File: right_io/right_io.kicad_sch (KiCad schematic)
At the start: 0 parts

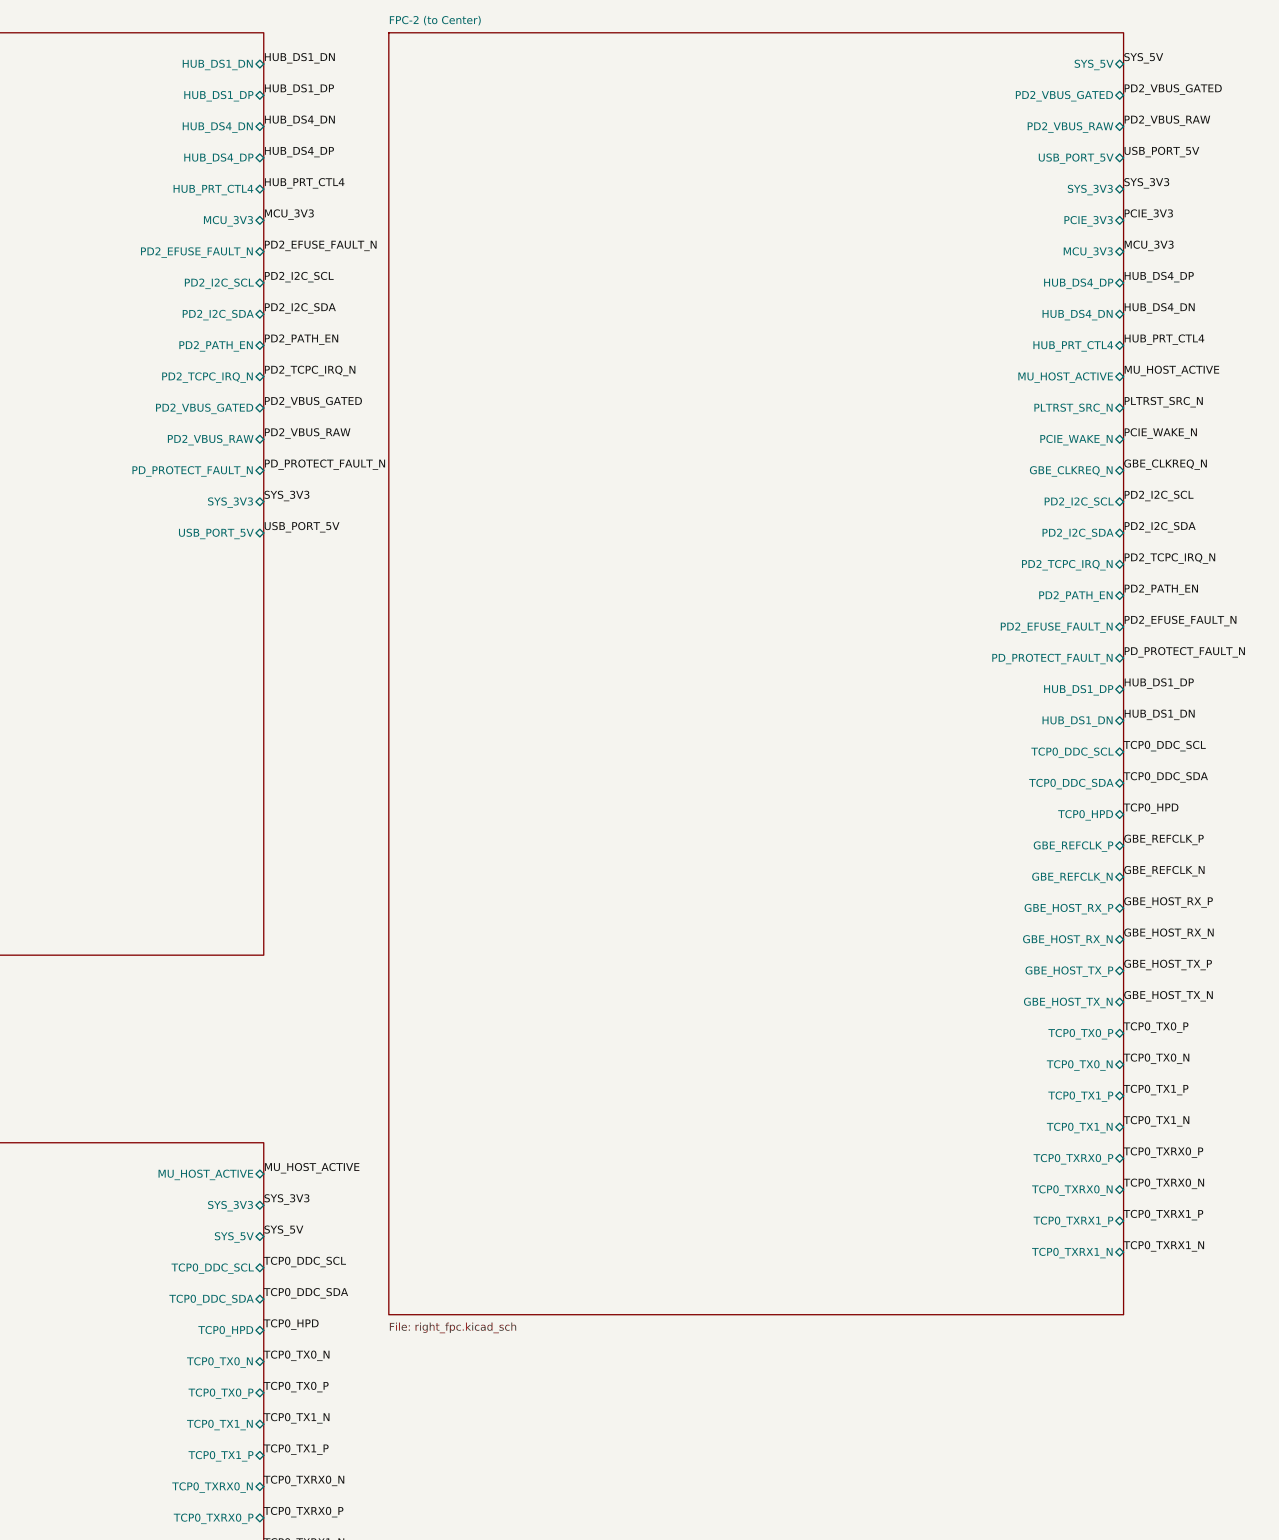
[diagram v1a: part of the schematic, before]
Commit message: fix the center layout and more board issues
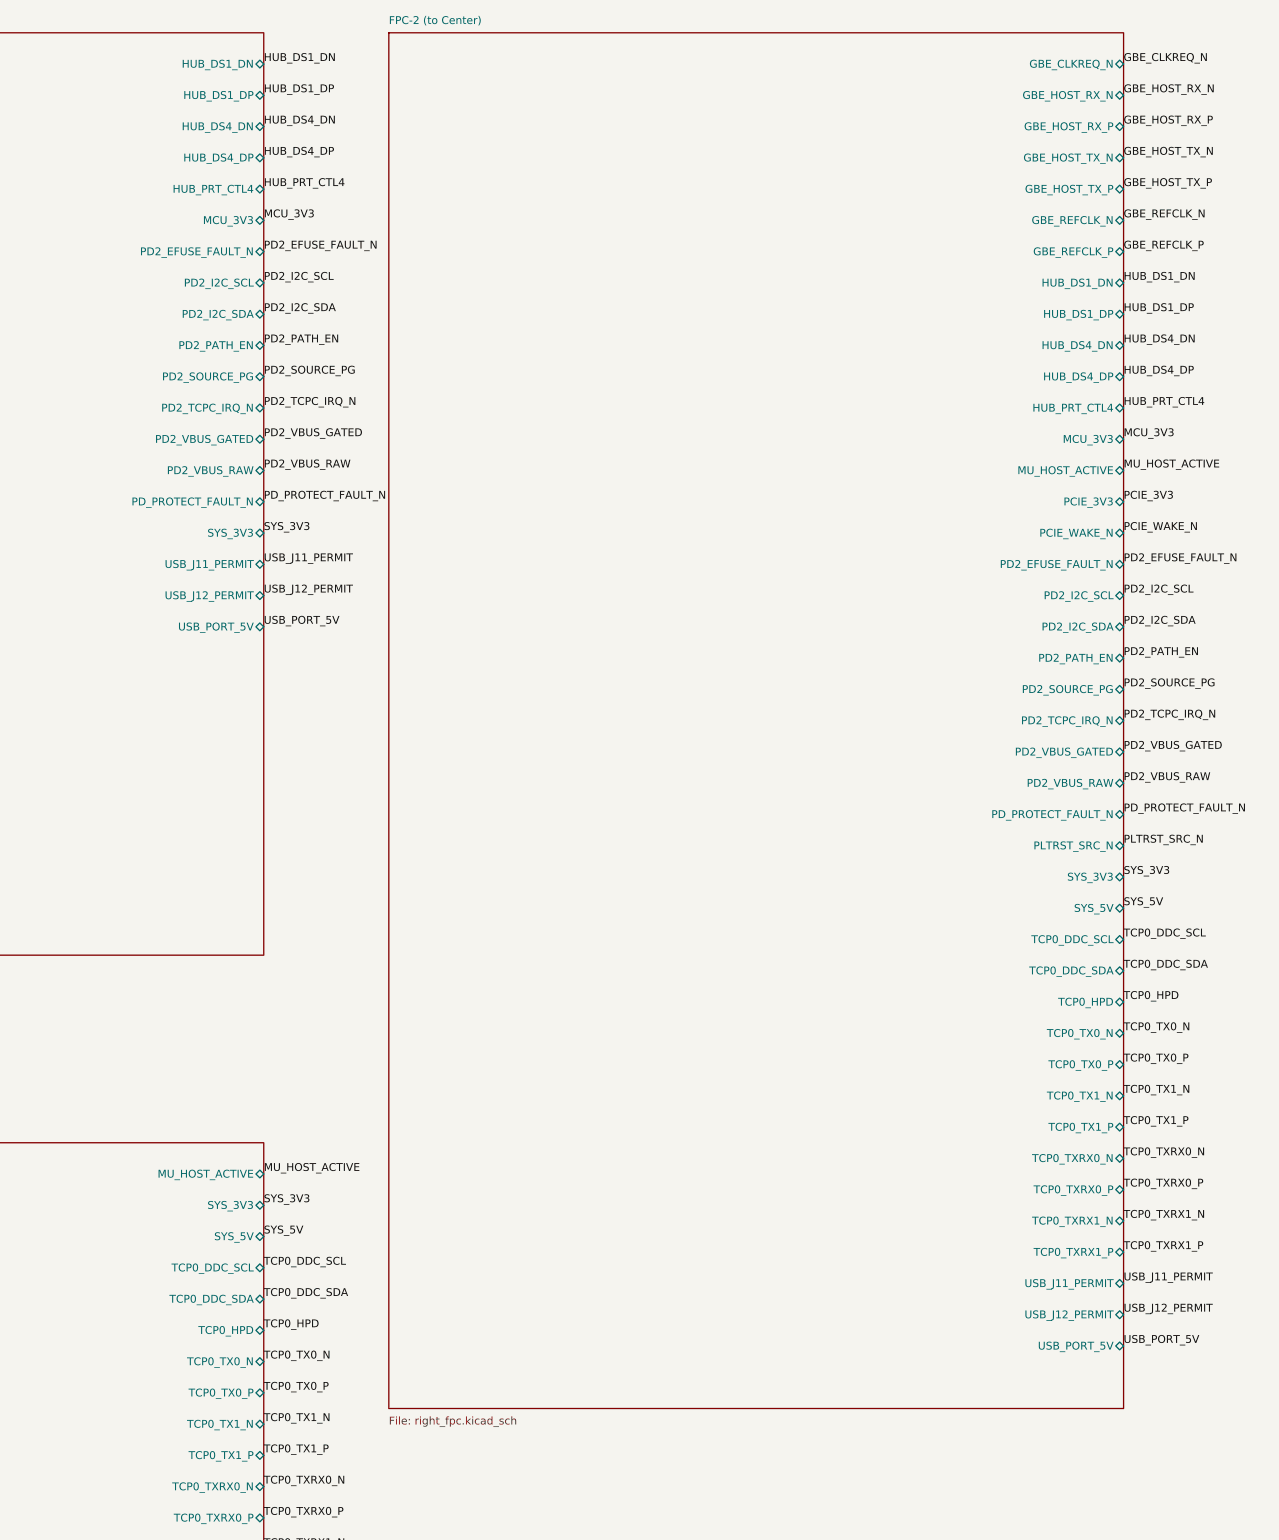
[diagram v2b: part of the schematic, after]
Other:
- sheet FPC-2 (to Center) ports: added PD2_SOURCE_PG, USB_J11_PERMIT, USB_J12_PERMIT; removed none
- sheet PD2 Dual-Role ports: added PD2_SOURCE_PG, USB_J11_PERMIT, USB_J12_PERMIT; removed none
